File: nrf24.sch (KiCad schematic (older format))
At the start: 2 parts, among them J1 Conn_01x08

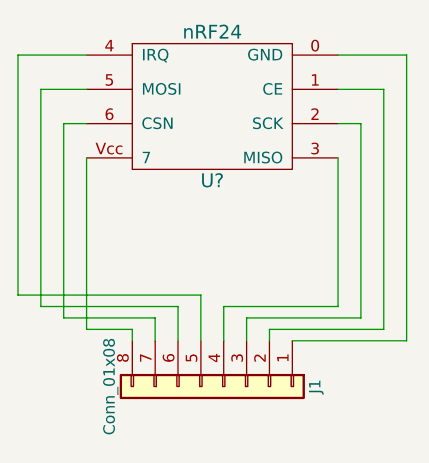
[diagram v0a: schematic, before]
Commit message: Initial layout
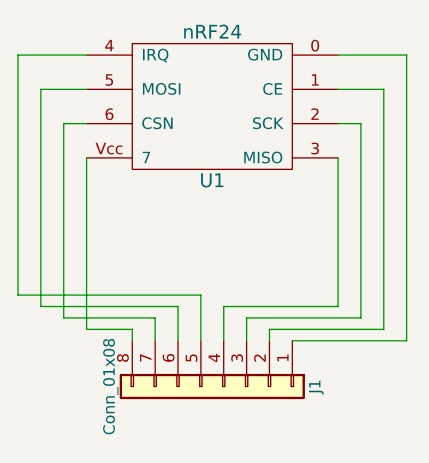
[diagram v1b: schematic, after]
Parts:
- U1: renamed from U?; footprint (none) -> nrf_footprints:nrf24_footprint
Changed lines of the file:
@@
 	5600 4450 5600 4650
 $Comp
-L nRF24 U?
+L nRF24 U1
 U 1 1 5A2E002F
 P 5650 3650
-F 0 "U?" H 5650 3350 60  0000 C CNN
+F 0 "U1" H 5650 3350 60  0000 C CNN
 F 1 "nRF24" H 5650 4000 60  0000 C CNN
-F 2 "" H 5650 3650 60  0001 C CNN
+F 2 "nrf_footprints:nrf24_footprint" H 5650 3650 60  0001 C CNN
 F 3 "" H 5650 3650 60  0001 C CNN
 	1    5650 3650

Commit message: final layout and gerber files
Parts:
- added C1: 10uF, Capacitors_THT:CP_Radial_D10.0mm_P5.00mm, symbol CP
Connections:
- wire segments 29 -> 31
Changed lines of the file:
@@
 LIBS:valves
 LIBS:nrf24_schematic_library
-LIBS:nrf24-cache
 EELAYER 25 0
 EELAYER END
@@
 	1    0    0    -1
 $EndComp
+$Comp
+L CP C1
+U 1 1 5A2F5C2C
+P 5600 4250
+F 0 "C1" H 5625 4350 50  0000 L CNN
+F 1 "10uF" H 5625 4150 50  0000 L CNN
+F 2 "Capacitors_THT:CP_Radial_D10.0mm_P5.00mm" H 5638 4100 50  0001 C CNN
+F 3 "" H 5600 4250 50  0001 C CNN
+	1    5600 4250
+	0    -1   -1   0
+$EndComp
+Wire Wire Line
+	5750 4250 6500 4250
+Connection ~ 6500 4250
+Wire Wire Line
+	5450 4250 5100 4250
+Connection ~ 5100 4250
 $EndSCHEMATC
